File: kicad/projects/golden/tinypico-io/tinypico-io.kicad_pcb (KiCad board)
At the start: 2 copper layers, 38.1 x 38.1 mm, 5 parts, among them J1 S2B-PH-SM4-TB(LF)(SN), J2 SM03B-SRSS-TB(LF)(SN), J3 SM04B-SRSS-TB(LF)(SN), J4 TSM-104-01-L-SV, J5 TSM-110-01-L-SV

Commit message: golden tinypico-io update pcb from schematic
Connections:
- net +3V3 renamed Net-(J3-Pad2)

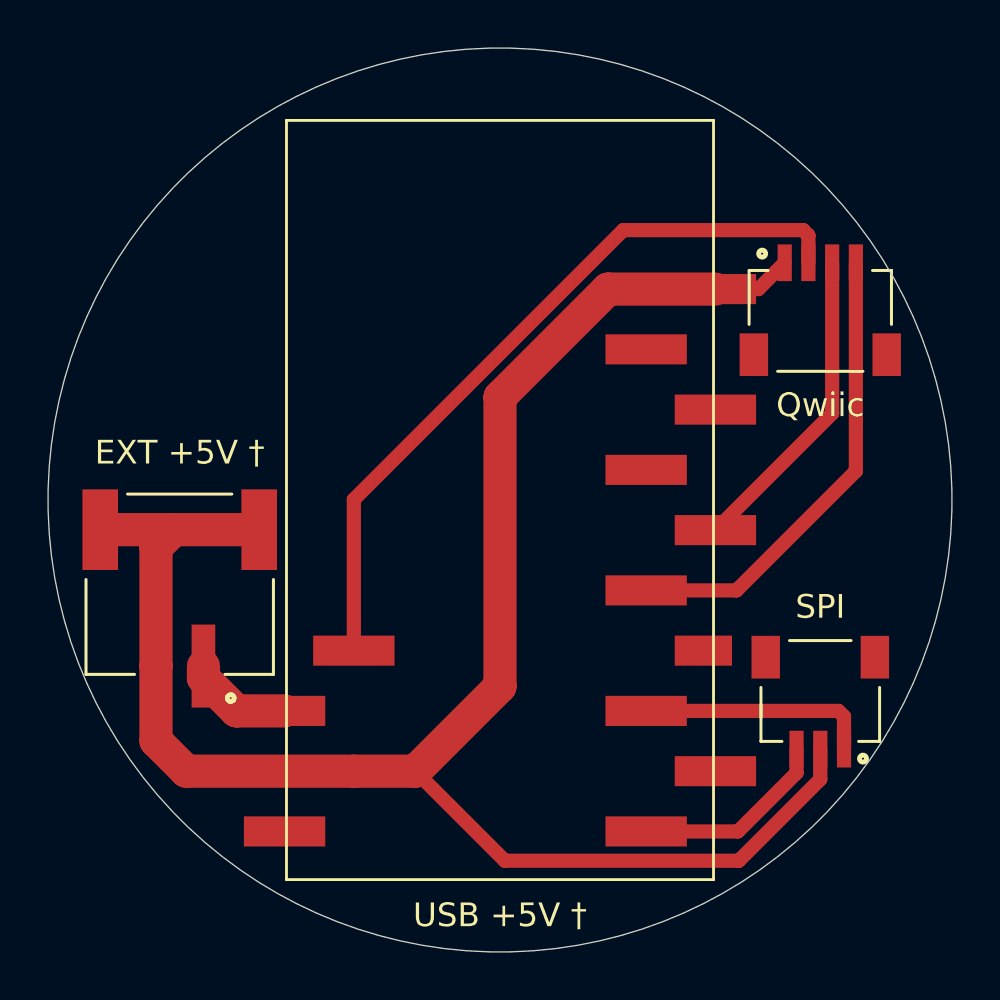
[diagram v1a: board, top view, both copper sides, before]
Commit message: golden tinypico-io version 1.0.0
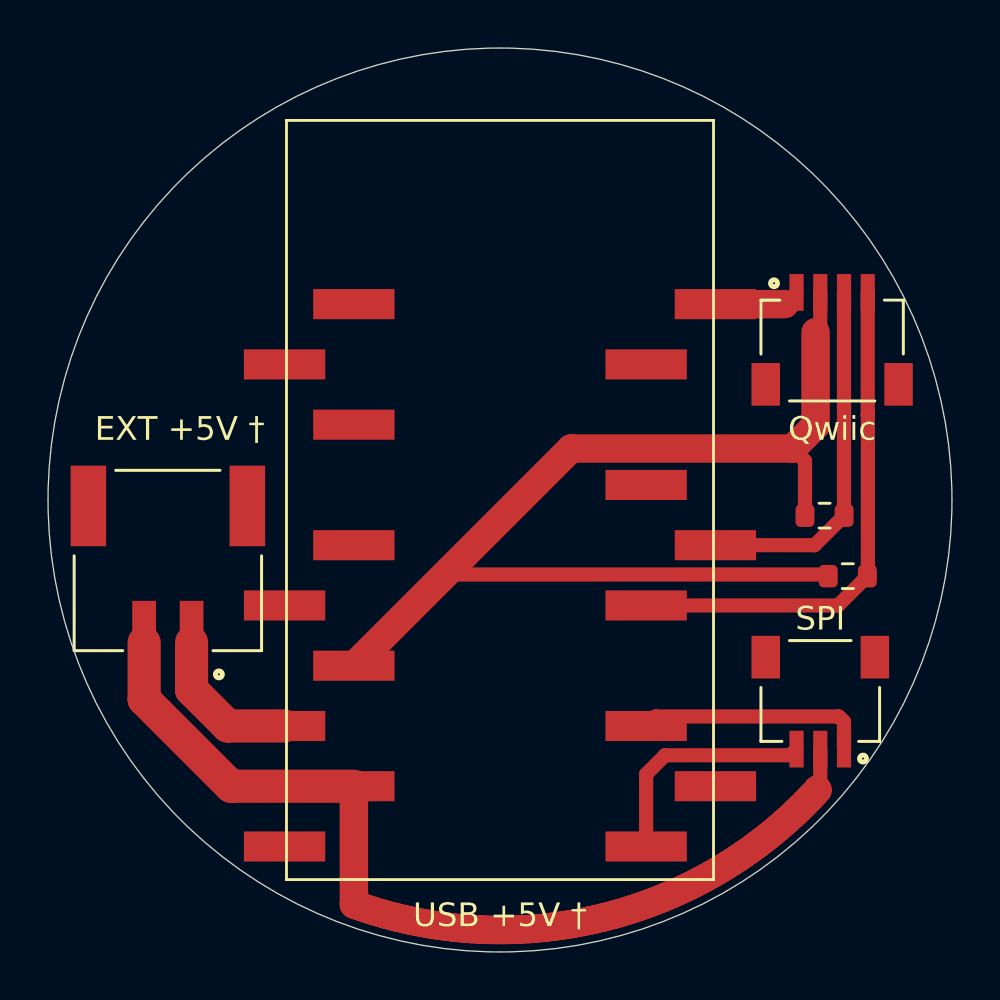
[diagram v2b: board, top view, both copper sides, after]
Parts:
- removed J4: TSM-104-01-L-SV, snapeda:TSM-104-01-L-SV
- removed J5: TSM-110-01-L-SV, snapeda:TSM-110-01-L-SV
- added R1: 1K, Resistor_SMD:R_0603_1608Metric, F.Cu at (163.7, 90.7)
- added R2: 1K, Resistor_SMD:R_0603_1608Metric, F.Cu at (164.7, 93.2)
- added U1: TinyPICO, tinypico-io:TinyPICO, F.Cu at (150.0, 90.0)
- moved J3 1.35 mm to (164.0, 81.2)
- moved J1 1.12 mm to (136.0, 96.0)
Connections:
- J1 pad S1: GND -> (no net)
- J1 pad S2: GND -> (no net)
- J2 pad S1: Net-(J2-PadS1) -> (no net)
- J2 pad S2: Net-(J2-PadS2) -> (no net)
- J3 pad 1: GND -> GND1
- J3 pad 2: Net-(J3-Pad2) -> /3V3
- J3 pad S1: Net-(J3-PadS1) -> (no net)
- J3 pad S2: Net-(J3-PadS2) -> (no net)
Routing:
- net /3V3: track 0.00 -> 59.3 mm
- net GND: track 80.3 -> 40.9 mm
- net Net-(J3-Pad2): track 31.5 -> 0.00 mm
- net GND1: track 0.00 -> 3.63 mm
- net SCL: track 19.7 -> 22.0 mm
- net +5V: track 4.50 -> 6.55 mm
- net SDA: track 13.3 -> 15.4 mm
- net MOSI: track 8.36 -> 9.83 mm
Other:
- board text added: "Provision by Wi-Fi AP ESP_«MAC address suffix» https://192.168.4.1/ Configure by either http://«mDNS hostname» http://«DHCP IP address»"
- board text added: "φ ArtLight Golden TinyPICO IO ©2021 Ross Tyler Version 1.0.0"
- board text removed: "φ ArtLight Golden TinyPICO IO ©2021 Ross Tyler"

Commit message: golden tinypico-io footprint fixes
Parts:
- U1: value TinyPICO -> TSM-110-01-L-SV
